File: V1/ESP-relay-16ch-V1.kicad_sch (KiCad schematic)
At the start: 145 parts, among them J1 +24VDC, J10 OUT7, J11 OUT8, J2 INPUTS, J3 USB_B_Micro, J4 OUT1, J5 OUT2, J6 OUT3, J7 OUT4, J8 OUT5, J9 OUT6, K1 G5PZ-1A, K2 G5PZ-1A, K3 G5PZ-1A, K4 G5PZ-1A, K5 G5PZ-1A, K6 G5PZ-1A, K7 G5PZ-1A, K8 G5PZ-1A, Q1 MMBT2222A/SOT-23-3, Q2 MMBT2222A/SOT-23-3, Q3 MMBT2222A/SOT-23-3, Q4 MMBT2222A/SOT-23-3, Q5 MMBT2222A/SOT-23-3, Q6 MMBT2222A/SOT-23-3, Q7 MMBT2222A/SOT-23-3, Q8 MMBT2222A/SOT-23-3, U1 SY8089A1AAC, U10 LTV-817S, U2 TX4138, U3 LTV-817S, U4 LTV-817S, U5 LTV-817S, U6 LTV-817S, U7 LTV-817S, U8 LTV-817S, U9 LTV-817S

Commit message: Development continues
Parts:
- removed C10, C11, C12, C5, C6, C7, C8, C9: 33nF/50V/0805, Tales:C_0805_2012Metric, symbol Device:C_Small
- removed D12, D13, D14, D15, D21, D22, D23, D24: BLUE/0603, Tales:LED_0603_1608Metric, symbol Device:LED_Small
- removed D16, D17, D18, D19, D26, D27, D28, D29: 1N4148/SOD-123, Tales:D_SOD-123, symbol Device:D_Small
- removed D2, D3, D4, D5, D6, D7, D8, D9: 9V1/500mW, Tales:D_MiniMELF, symbol Device:D_Zener_Small
- removed D20: B5819W, Tales:D_SOD-123, symbol Device:D_Schottky_Small
- removed D25, D30, D31: GREEN/0603, Tales:LED_0603_1608Metric, symbol Device:LED_Small
- removed J10: OUT7, Tales:TerminalBlock_Phoenix_MKDS-3-2-5.08_1x02_P5.08mm_Horizontal, symbol Connector_Generic:Conn_01x02
- removed J11: OUT8, Tales:TerminalBlock_Phoenix_MKDS-3-2-5.08_1x02_P5.08mm_Horizontal, symbol Connector_Generic:Conn_01x02
- removed J4: OUT1, Tales:TerminalBlock_Phoenix_MKDS-3-2-5.08_1x02_P5.08mm_Horizontal, symbol Connector_Generic:Conn_01x02
- removed J5: OUT2, Tales:TerminalBlock_Phoenix_MKDS-3-2-5.08_1x02_P5.08mm_Horizontal, symbol Connector_Generic:Conn_01x02
- removed J6: OUT3, Tales:TerminalBlock_Phoenix_MKDS-3-2-5.08_1x02_P5.08mm_Horizontal, symbol Connector_Generic:Conn_01x02
- removed J7: OUT4, Tales:TerminalBlock_Phoenix_MKDS-3-2-5.08_1x02_P5.08mm_Horizontal, symbol Connector_Generic:Conn_01x02
- removed J8: OUT5, Tales:TerminalBlock_Phoenix_MKDS-3-2-5.08_1x02_P5.08mm_Horizontal, symbol Connector_Generic:Conn_01x02
- removed J9: OUT6, Tales:TerminalBlock_Phoenix_MKDS-3-2-5.08_1x02_P5.08mm_Horizontal, symbol Connector_Generic:Conn_01x02
- removed K1, K2, K3, K4, K5, K6, K7, K8: G5PZ-1A, Tales:Relay_SPST_Omron-G5PZ-1A, symbol Tales:G5PZ-1A
- removed Q1, Q2, Q3, Q4, Q5, Q6, Q7, Q8: MMBT2222A/SOT-23-3, Tales:SOT-23, symbol Device:Q_NPN_BEC
- removed R10, R3, R4, R5, R6, R7, R8, R9: 1k2/0,125W/0805, Tales:R_0805_2012Metric, symbol Device:R_US
- removed R13, R14, R15, R16, R17, R18, R19, R20: 3k3/0,125W/0805, Tales:R_0805_2012Metric, symbol Device:R_US
- removed R23, R25, R27, R29, R35, R37, R39, R41: 4k7/0,125W/0805, Tales:R_0805_2012Metric, symbol Device:R_US
- removed R24, R26, R28, R30, R36, R38, R40, R42: 10k/0,125W/0805, Tales:R_0805_2012Metric, symbol Device:R_US
- removed R31, R32, R33, R34, R44, R45, R46, R47: 1k/0,125W/0805, Tales:R_0805_2012Metric, symbol Device:R_US
- removed RV1, RV2, RV3, RV4, RV5, RV6, RV7, RV8: 250VAC, Tales:RV_Disc_D12mm_W3.9mm_P7.5mm, symbol Device:Varistor
- removed U10, U3, U4, U5, U6, U7, U8, U9: LTV-817S, Package_DIP:SMDIP-4_W9.53mm, symbol Isolator:LTV-817S
- added C?: 10uF/16V/1206, Tales:C_1206_3216Metric, symbol Device:C_Polarized_Small_US
- added C?: 0,1uF/50V/0805, Tales:C_0805_2012Metric, symbol Device:C_Small
- added D? (x3): BLUE/0603, Tales:LED_0603_1608Metric, symbol Device:LED_Small
- added D?: B5819W, Tales:D_SOD-123, symbol Device:D_Schottky_Small
- added J4: RJ45, Connector_RJ:RJ45_Amphenol_RJHSE5380, symbol Connector:RJ45
- added J5: OUTPUTS, symbol Connector_Generic:Conn_01x18
- added Q1: UMH3N, Package_TO_SOT_SMD:SOT-363_SC-70-6, symbol Transistor_BJT:UMH3N
- added R? (x2): 10k/0,125W/0805, Tales:R_0805_2012Metric, symbol Device:R_US
- added R?: 470R/0,125W/0805, Tales:R_0805_2012Metric, symbol Device:R_US
- added U3: CH340C, Package_SO:SOIC-16_3.9x9.9mm_P1.27mm, symbol Interface_USB:CH340C
- added U4: LAN8710A, Package_DFN_QFN:QFN-32-1EP_5x5mm_P0.5mm_EP3.3x3.3mm_ThermalVias, symbol Interface_Ethernet:LAN8710A
- added U5, U?: PCF8574, Tales:SO-16_7.5x10.3mm_P1.27mm, symbol Interface_Expansion:PCF8574
- added U6: ESP32-WROOM-32, RF_Module:ESP32-WROOM-32, symbol RF_Module:ESP32-WROOM-32
- J2: symbol Connector_Generic:Conn_01x08 -> Connector_Generic:Conn_01x16
- renumbered U2 to U1, U1 to U2
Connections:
- net +VReg is gone; now on net +24V: C3.1, C4.1, D1.1 (K), R11.1, R43.1, U1.3 (VIN)
- net +24V: now also J5.1 (Pin_1), J5.18 (Pin_18); no longer D1.2 (A), J1.1 (Pin_1)
- net +3.3V: now also C?.1, C?.1, R?.1, R?.1, U3.16 (VCC), U3.4 (V3), U6.2 (VDD)
- net GNDREF: now also C?.2, C?.2, D?.1 (K), D?.1 (K), D?.1 (K), U3.1 (GND), U6.1 (GND), U6.15 (GND), U6.38 (GND), U6.39 (GND)
- net J2-IN1: now reaches J2.1 (Pin_1)
- net at R43.2: now also D?.2 (A)
- net J2-IN2: now reaches J2.2 (Pin_2)
- net J2-IN3: now reaches J2.3 (Pin_3)
- net J2-IN4: now reaches J2.4 (Pin_4)
- net J2-IN5: now reaches J2.5 (Pin_5)
- net J2-IN6: now reaches J2.6 (Pin_6)
- net J2-IN7: now reaches J2.7 (Pin_7)
- net J2-IN8: now reaches J2.8 (Pin_8)
- net at R48.2: now also D?.2 (A)
- net at R49.2: now also D?.2 (A)
- net at F1.1: now also D?.1 (K)
- net at J3.1 (VBUS): now also D?.2 (A)
- net D+: no longer names the net of J3.3 (D+)
- net D+: now also U3.5 (UD+)
- net D-: no longer names the net of J3.2 (D-)
- net D-: now also U3.6 (UD-)
- new net: D1.2 (A), J1.1 (Pin_1)
- new net: Q1.2 (B1), Q1.4 (E2), U3.13 (~{DTR})
- new net: Q1.1 (E1), Q1.5 (B2), U3.14 (~{RTS})
- new net: U3.2 (TXD), U6.34 (RXD0/IO3)
- new net: R?.2, U3.3 (RXD)
- new net: Q1.6 (C1), R?.2, U6.3 (EN)
- new net: Q1.3 (C2), R?.2, U6.25 (IO0)
- new net: R?.1, U6.35 (TXD0/IO1)
- new net J2-IN10: J2.10 (Pin_10)
- new net J2-IN11: J2.11 (Pin_11)
- new net J2-IN12: J2.12 (Pin_12)
- new net J2-IN13: J2.13 (Pin_13)
- new net J2-IN14: J2.14 (Pin_14)
- new net J2-IN15: J2.15 (Pin_15)
- new net J2-IN16: J2.16 (Pin_16)
- new net J2-IN9: J2.9 (Pin_9)
- new net J5-OUT1: J5.2 (Pin_2)
- new net J5-OUT10: J5.11 (Pin_11)
- new net J5-OUT11: J5.12 (Pin_12)
- new net J5-OUT12: J5.13 (Pin_13)
- new net J5-OUT13: J5.14 (Pin_14)
- new net J5-OUT14: J5.15 (Pin_15)
- new net J5-OUT15: J5.16 (Pin_16)
- new net J5-OUT16: J5.17 (Pin_17)
- new net J5-OUT2: J5.3 (Pin_3)
- new net J5-OUT3: J5.4 (Pin_4)
- new net J5-OUT4: J5.5 (Pin_5)
- new net J5-OUT5: J5.6 (Pin_6)
- new net J5-OUT6: J5.7 (Pin_7)
- new net J5-OUT7: J5.8 (Pin_8)
- new net J5-OUT8: J5.9 (Pin_9)
- new net J5-OUT9: J5.10 (Pin_10)
- no-connect marks 3 -> 8
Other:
- removed sheet ESP32
- added sheet Inputs (ESP-relay-16ch-V1-inputs.kicad_sch)
- added sheet Outputs (ESP-relay-16ch-V1-outputs.kicad_sch)
- moved on the sheet: C1, C13, C14, C15, C16, C2, C3, C4, D1, D10, D11, L1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

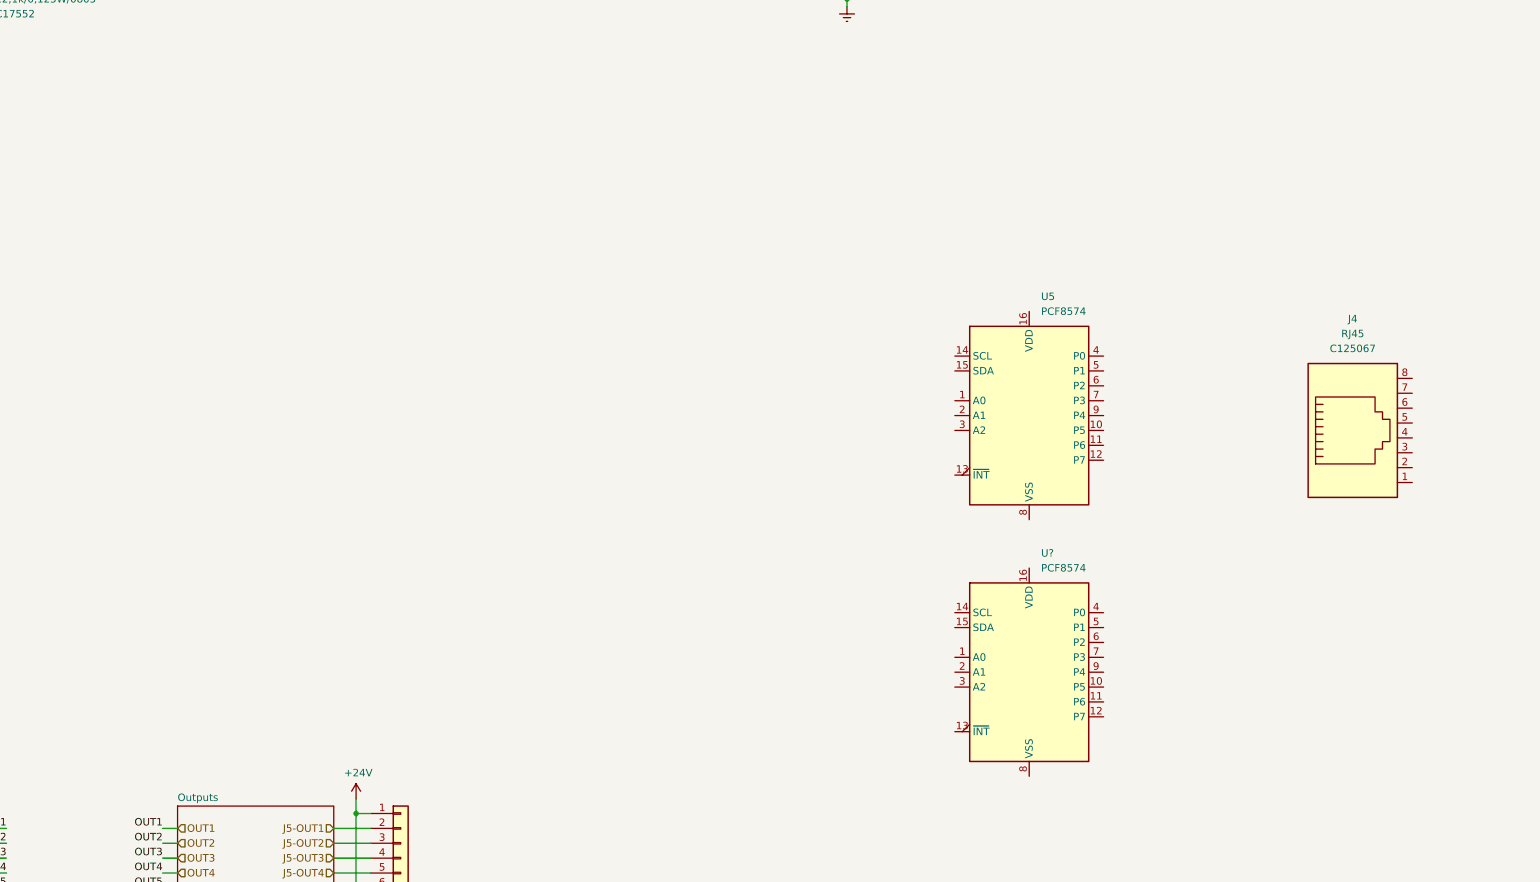
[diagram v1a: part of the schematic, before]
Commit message: Update ESP-relay-16ch-V1.kicad_sch
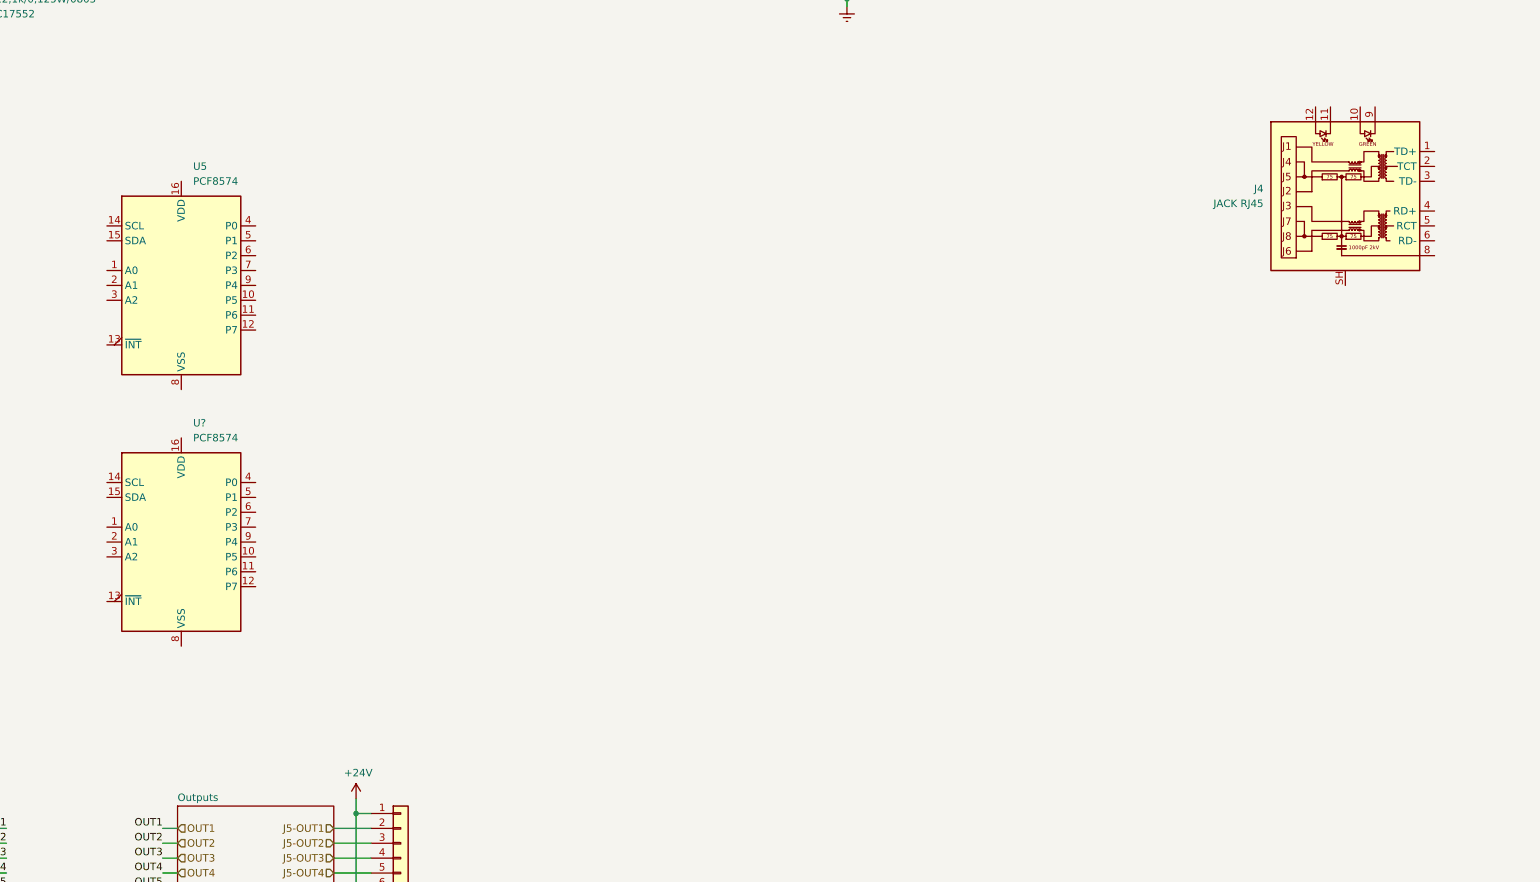
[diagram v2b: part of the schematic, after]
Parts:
- removed J4: RJ45, Connector_RJ:RJ45_Amphenol_RJHSE5380, symbol Connector:RJ45
- added J4: JACK RJ45, symbol Tales:HanRun HR913550A
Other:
- moved on the sheet: U5, U?
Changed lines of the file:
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@@
     (pin "2")
   )
-  (symbol (lib_id "Interface_Expansion:PCF8574") (at 245.745 163.83 0) (unit 1)
+  (symbol (lib_id "Interface_Expansion:PCF8574") (at 100.965 141.605 0) (unit 1)
     (in_bom yes) (on_board yes) (fields_autoplaced)
-    (property "Reference" "U5" (id 0) (at 247.7644 143.51 0)
-      (effects (font (size 1.27 1.27)) (justify left))
-    )
-    (property "Value" "PCF8574" (id 1) (at 247.7644 146.05 0)
-      (effects (font (size 1.27 1.27)) (justify left))
-    )
-    (property "Footprint" "Tales:SO-16_7.5x10.3mm_P1.27mm" (id 2) (at 245.745 163.83 0)
-      (effects (font (size 1.27 1.27)) hide)
-    )
-    (property "Datasheet" "http://www.nxp.com/documents/data_sheet/PCF8574_PCF8574A.pdf" (id 3) (at 245.745 163.83 0)
+    (property "Reference" "U5" (id 0) (at 102.9844 121.285 0)
+      (effects (font (size 1.27 1.27)) (justify left))
+    )
+    (property "Value" "PCF8574" (id 1) (at 102.9844 123.825 0)
+      (effects (font (size 1.27 1.27)) (justify left))
+    )
+    (property "Footprint" "Tales:SO-16_7.5x10.3mm_P1.27mm" (id 2) (at 100.965 141.605 0)
+      (effects (font (size 1.27 1.27)) hide)
+    )
+    (property "Datasheet" "http://www.nxp.com/documents/data_sheet/PCF8574_PCF8574A.pdf" (id 3) (at 100.965 141.605 0)
       (effects (font (size 1.27 1.27)) hide)
     )
@@
     (pin "2")
   )
-  (symbol (lib_id "Connector:RJ45") (at 300.99 167.64 0) (unit 1)
-    (in_bom yes) (on_board yes)
-    (property "Reference" "J4" (id 0) (at 300.99 147.32 0))
-    (property "Value" "RJ45" (id 1) (at 300.99 149.86 0))
-    (property "Footprint" "Connector_RJ:RJ45_Amphenol_RJHSE5380" (id 2) (at 300.99 167.005 90)
-      (effects (font (size 1.27 1.27)) hide)
-    )
-    (property "Datasheet" "~" (id 3) (at 300.99 167.005 90)
-      (effects (font (size 1.27 1.27)) hide)
-    )
-    (property "Case" "~" (id 4) (at 300.99 167.64 0)
-      (effects (font (size 1.27 1.27)) hide)
-    )
-    (property "JLCPCB BOM" "1" (id 5) (at 300.99 167.64 0)
-      (effects (font (size 1.27 1.27)) hide)
-    )
-    (property "LCSC Part #" "C125067" (id 6) (at 300.99 152.4 0))
-    (property "Mfr" "TE Connectivity" (id 7) (at 300.99 167.64 0)
-      (effects (font (size 1.27 1.27)) hide)
-    )
-    (property "Mfr PN" "1-406541-1" (id 8) (at 300.99 167.64 0)
-      (effects (font (size 1.27 1.27)) hide)
-    )
-    (property "Technology" "~" (id 9) (at 300.99 167.64 0)
-      (effects (font (size 1.27 1.27)) hide)
-    )
-    (property "Vendor" "JLCPCB" (id 10) (at 300.99 167.64 0)
-      (effects (font (size 1.27 1.27)) hide)
-    )
-    (property "Vendor PN" "C125067" (id 11) (at 300.99 167.64 0)
-      (effects (font (size 1.27 1.27)) hide)
-    )
-    (pin "1")
-    (pin "2")
-    (pin "3")
-    (pin "4")
-    (pin "5")
-    (pin "6")
-    (pin "7")
-    (pin "8")
-  )
   (symbol (lib_id "power:GNDREF") (at 34.925 83.82 0) (unit 1)
     (in_bom yes) (on_board yes)
@@
     (pin "2")
   )
-  (symbol (lib_id "Interface_Expansion:PCF8574") (at 245.745 207.645 0) (unit 1)
+  (symbol (lib_id "Interface_Expansion:PCF8574") (at 100.965 185.42 0) (unit 1)
     (in_bom yes) (on_board yes) (fields_autoplaced)
-    (property "Reference" "U?" (id 0) (at 247.7644 187.325 0)
-      (effects (font (size 1.27 1.27)) (justify left))
-    )
-    (property "Value" "PCF8574" (id 1) (at 247.7644 189.865 0)
-      (effects (font (size 1.27 1.27)) (justify left))
-    )
-    (property "Footprint" "Tales:SO-16_7.5x10.3mm_P1.27mm" (id 2) (at 245.745 207.645 0)
-      (effects (font (size 1.27 1.27)) hide)
-    )
-    (property "Datasheet" "http://www.nxp.com/documents/data_sheet/PCF8574_PCF8574A.pdf" (id 3) (at 245.745 207.645 0)
+    (property "Reference" "U?" (id 0) (at 102.9844 165.1 0)
+      (effects (font (size 1.27 1.27)) (justify left))
+    )
+    (property "Value" "PCF8574" (id 1) (at 102.9844 167.64 0)
+      (effects (font (size 1.27 1.27)) (justify left))
+    )
+    (property "Footprint" "Tales:SO-16_7.5x10.3mm_P1.27mm" (id 2) (at 100.965 185.42 0)
+      (effects (font (size 1.27 1.27)) hide)
+    )
+    (property "Datasheet" "http://www.nxp.com/documents/data_sheet/PCF8574_PCF8574A.pdf" (id 3) (at 100.965 185.42 0)
       (effects (font (size 1.27 1.27)) hide)
     )
@@
     (pin "2")
   )
+  (symbol (lib_id "Tales:HanRun HR913550A") (at 299.72 126.365 0) (unit 1)
+    (in_bom yes) (on_board yes) (fields_autoplaced)
+    (property "Reference" "J4" (id 0) (at 285.75 125.0949 0)
+      (effects (font (size 1.27 1.27)) (justify right))
+    )
+    (property "Value" "JACK RJ45" (id 1) (at 285.75 127.6349 0)
+      (effects (font (size 1.27 1.27)) (justify right))
+    )
+    (property "Footprint" "" (id 2) (at 299.72 145.415 0)
+      (effects (font (size 1.27 1.27)) hide)
+    )
+    (property "Datasheet" "" (id 3) (at 289.179 132.334 0)
+      (effects (font (size 1.27 1.27)) (justify left top) hide)
+    )
+    (pin "1")
+    (pin "10")
+    (pin "11")
+    (pin "12")
+    (pin "2")
+    (pin "3")
+    (pin "4")
+    (pin "5")
+    (pin "6")
+    (pin "8")
+    (pin "9")
+    (pin "SH")
+  )
   (symbol (lib_id "power:GNDREF") (at 92.075 83.82 0) (unit 1)
     (in_bom yes) (on_board yes)
@@
       (reference "J3") (unit 1) (value "USB_B_Micro") (footprint "Connector_USB:USB_Micro-B_Amphenol_10118194_Horizontal")
     )
-    (path "/8d731b43-d84e-455f-843c-dcaec73c4937"
-      (reference "J4") (unit 1) (value "RJ45") (footprint "Connector_RJ:RJ45_Amphenol_RJHSE5380")
+    (path "/cc8a8574-e5fa-40ff-936b-4f2b5c6a6164"
+      (reference "J4") (unit 1) (value "JACK RJ45") (footprint "")
     )
     (path "/229e0179-2ec4-47b8-a4bf-44484ffd7818"
